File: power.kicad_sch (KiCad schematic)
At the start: 5 parts, among them U12 HX TYPE-C 6PIN

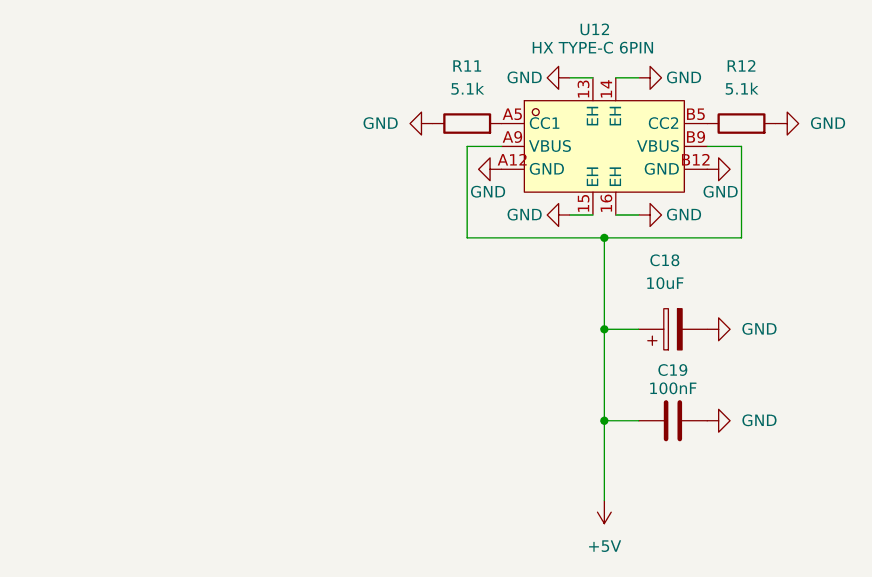
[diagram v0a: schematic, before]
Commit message: starting the layout
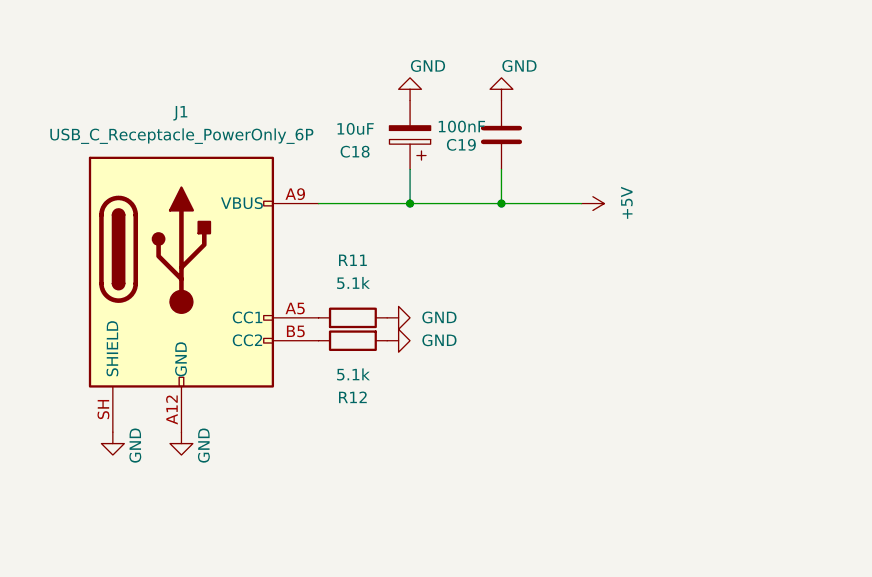
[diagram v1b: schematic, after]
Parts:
- removed U12: HX TYPE-C 6PIN, EasyEDA:USB-C-SMD_HX-TYPE-C-6PIN, symbol EasyEDA:HXTYPE-C6PIN
- added J1: USB_C_Receptacle_PowerOnly_6P, Connector_USB:USB_C_Receptacle_GCT_USB4105-xx-A_16P_TopMnt_Horizontal, symbol Connector:USB_C_Receptacle_PowerOnly_6P
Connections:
- net +5V: now also J1.A9 (VBUS), J1.B9 (VBUS)
- net GND: now also J1.A12 (GND), J1.B12 (GND), J1.SH (SHIELD)
- net at R11.2: now also J1.A5 (CC1)
- net at R12.1: now also J1.B5 (CC2)

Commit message: start to make the clk signal
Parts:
- J1: footprint Connector_USB:USB_C_Receptacle_GCT_USB4105-xx-A_16P_TopMnt_Horizontal -> Connector_USB:USB_C_Receptacle_GCT_USB4125-xx-x-0190_6P_TopMnt_Horizontal
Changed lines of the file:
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@@
 			)
 		)
-		(property "Footprint" "Connector_USB:USB_C_Receptacle_GCT_USB4105-xx-A_16P_TopMnt_Horizontal"
+		(property "Footprint" "Connector_USB:USB_C_Receptacle_GCT_USB4125-xx-x-0190_6P_TopMnt_Horizontal"
 			(at 43.18 95.25 0)
 			(hide yes)
